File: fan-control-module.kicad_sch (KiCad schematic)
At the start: 1 part

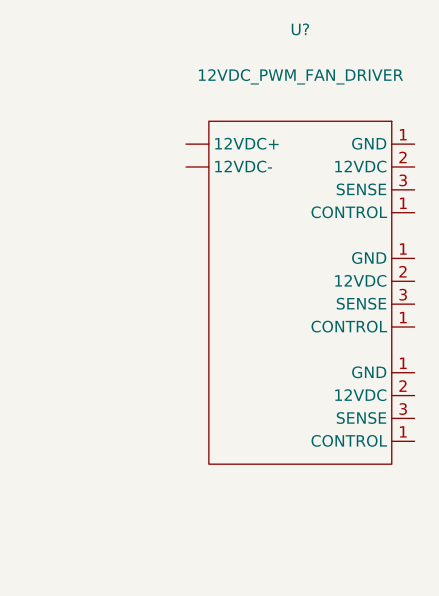
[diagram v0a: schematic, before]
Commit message: Bunch more changes
Blah blah
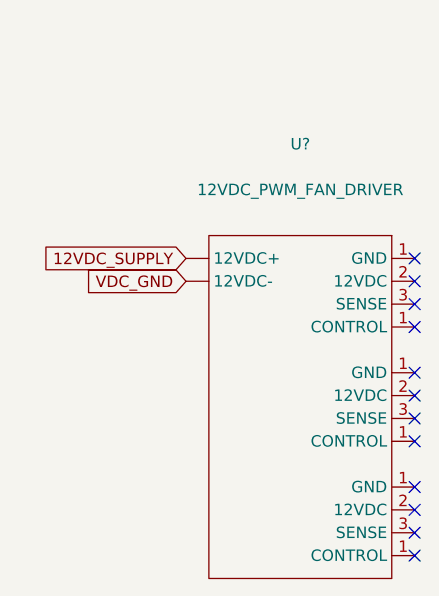
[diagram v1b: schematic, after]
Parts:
- removed U?: 12VDC_PWM_FAN_DRIVER, symbol bvm-library:12VDC_PWM_FAN_DRIVER
- added U?: 12VDC_PWM_FAN_DRIVER, symbol bvm-library:12VDC_PWM_FAN_DRIVER
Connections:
- new net 12VDC_SUPPLY: U?. (12VDC-)
- new net VDC_GND: U?. (12VDC-)
- no-connect marks 0 -> 12
